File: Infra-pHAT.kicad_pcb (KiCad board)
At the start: 2 copper layers, 65 x 30 mm, 25 parts, among them Q1 BC817, U1 CAT24C32WI-GT3

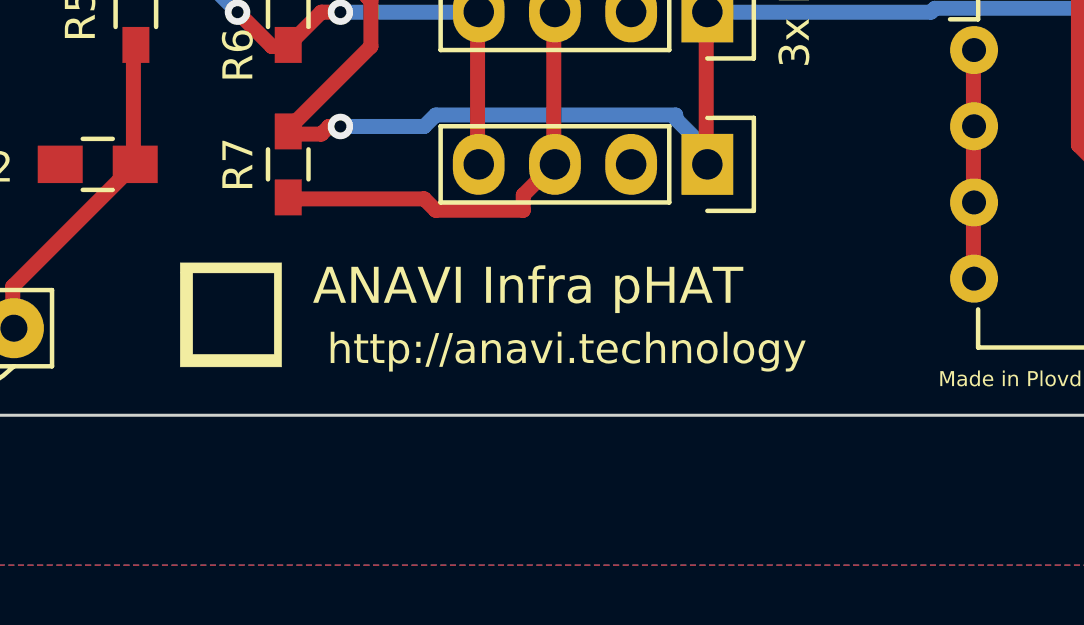
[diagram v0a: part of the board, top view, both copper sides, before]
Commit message: Infra-pHAT.kicad_pcb: Add revision number
Signed-off-by: Leon Anavi <leon@anavi.org>
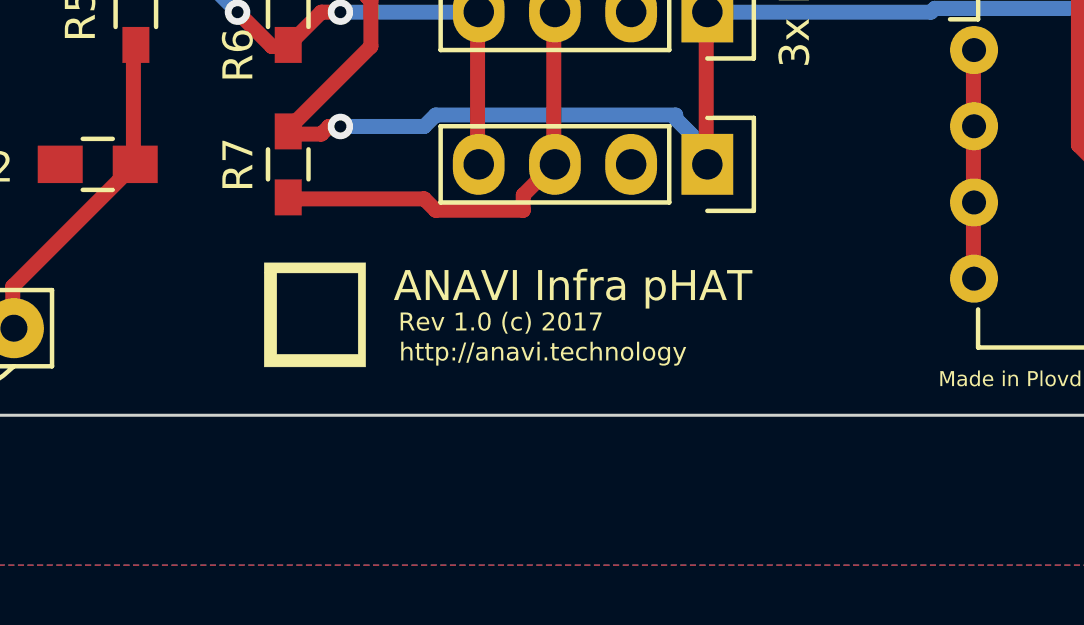
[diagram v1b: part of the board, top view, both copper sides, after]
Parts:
- moved ? 2.80 mm to (175.3, 101.7)
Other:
- board text added: "Rev 1.0 (c) 2017"
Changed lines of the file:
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@@
     (links 59)
     (no_connects 2)
-    (area 148.451099 74.953599 213.551101 105.053601)
+    (area 136.817429 66.3 225.182572 110.000001)
     (thickness 1.6)
-    (drawings 21)
+    (drawings 22)
     (tracks 236)
     (zones 0)
@@
     (pcbplotparams
       (layerselection 0x00030_80000001)
-      (usegerberextensions false)
+      (usegerberextensions true)
       (excludeedgelayer true)
       (linewidth 0.100000)
@@
       (outputformat 1)
       (mirror false)
-      (drillshape 1)
+      (drillshape 0)
       (scaleselection 1)
-      (outputdirectory ""))
+      (outputdirectory plots/))
   )
   (net 0 "")
@@
   )
   (module logo:anavi-logo (layer F.Cu)
-    (at 172.5 101.7)
+    (at 175.3 101.7)
     (fp_text reference "" (at 0 0) (layer F.SilkS) hide
       (effects (font (thickness 0.3)))
@@
       (xy -1.693333 -1.439333) (xy -1.693333 -1.778) (xy 1.693334 -1.778) (xy 1.693334 1.693334)) (layer F.SilkS) (width 0.01))
   )
+  (gr_text "Rev 1.0 (c) 2017" (at 181.5 101.9) (layer F.SilkS)
+    (effects (font (size 0.6 0.6) (thickness 0.15)))
+  )
   (gr_text "3.3V TX  RX GND" (at 170.9 83.9) (layer F.SilkS)
     (effects (font (size 0.8 0.8) (thickness 0.125)))
@@
     (effects (font (size 0.5 0.5) (thickness 0.125)))
   )
-  (gr_text http://anavi.technology (at 183.7 102.8) (layer F.SilkS)
-    (effects (font (size 1 1) (thickness 0.2)))
-  )
-  (gr_text "ANAVI Infra pHAT" (at 182.4 100.7) (layer F.SilkS)
-    (effects (font (size 1.2 1.2) (thickness 0.3)))
+  (gr_text http://anavi.technology (at 182.9 102.9) (layer F.SilkS)
+    (effects (font (size 0.6 0.6) (thickness 0.15)))
+  )
+  (gr_text "ANAVI Infra pHAT" (at 183.9 100.7) (layer F.SilkS)
+    (effects (font (size 1 1) (thickness 0.25)))
   )
   (dimension 3.5 (width 0.3) (layer F.CrtYd)
